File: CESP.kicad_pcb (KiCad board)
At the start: 2 copper layers, 55.9 x 44.7 mm, 9 parts

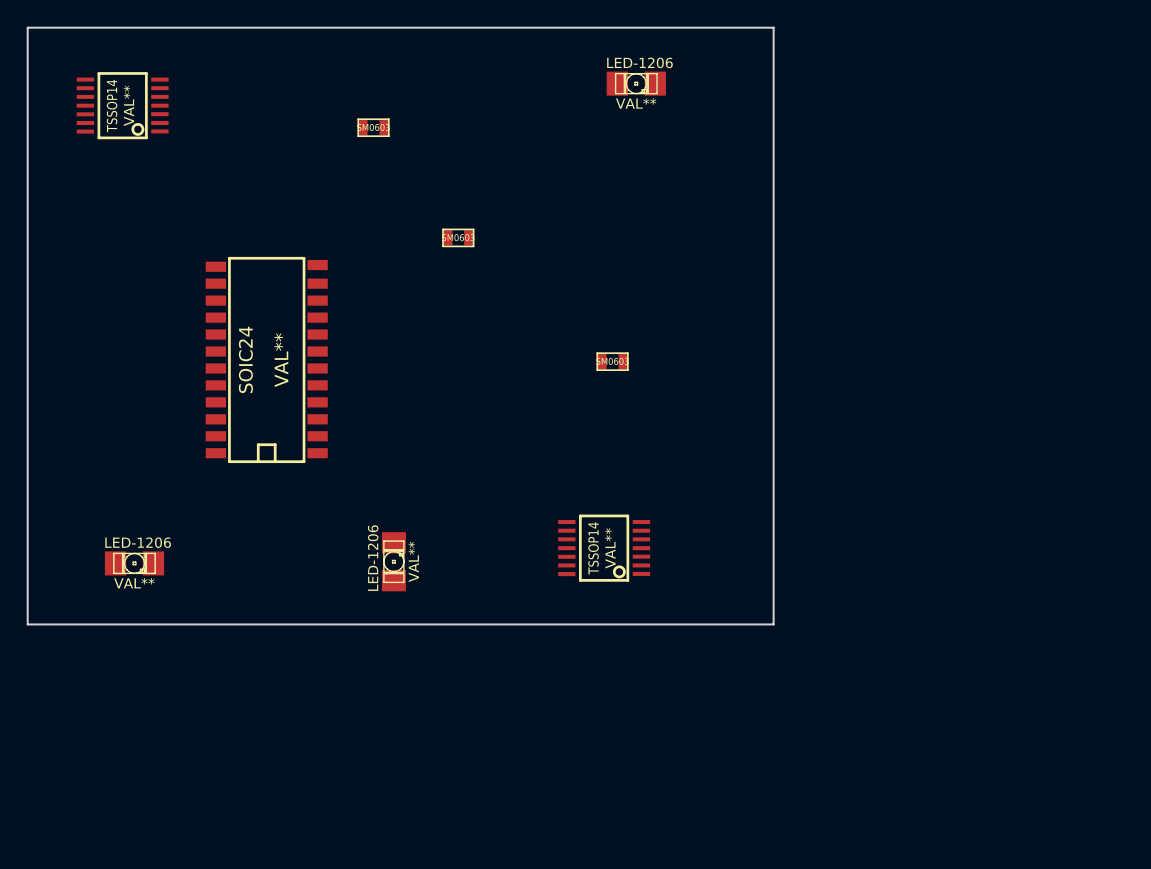
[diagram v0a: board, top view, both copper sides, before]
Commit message: Version1 commit
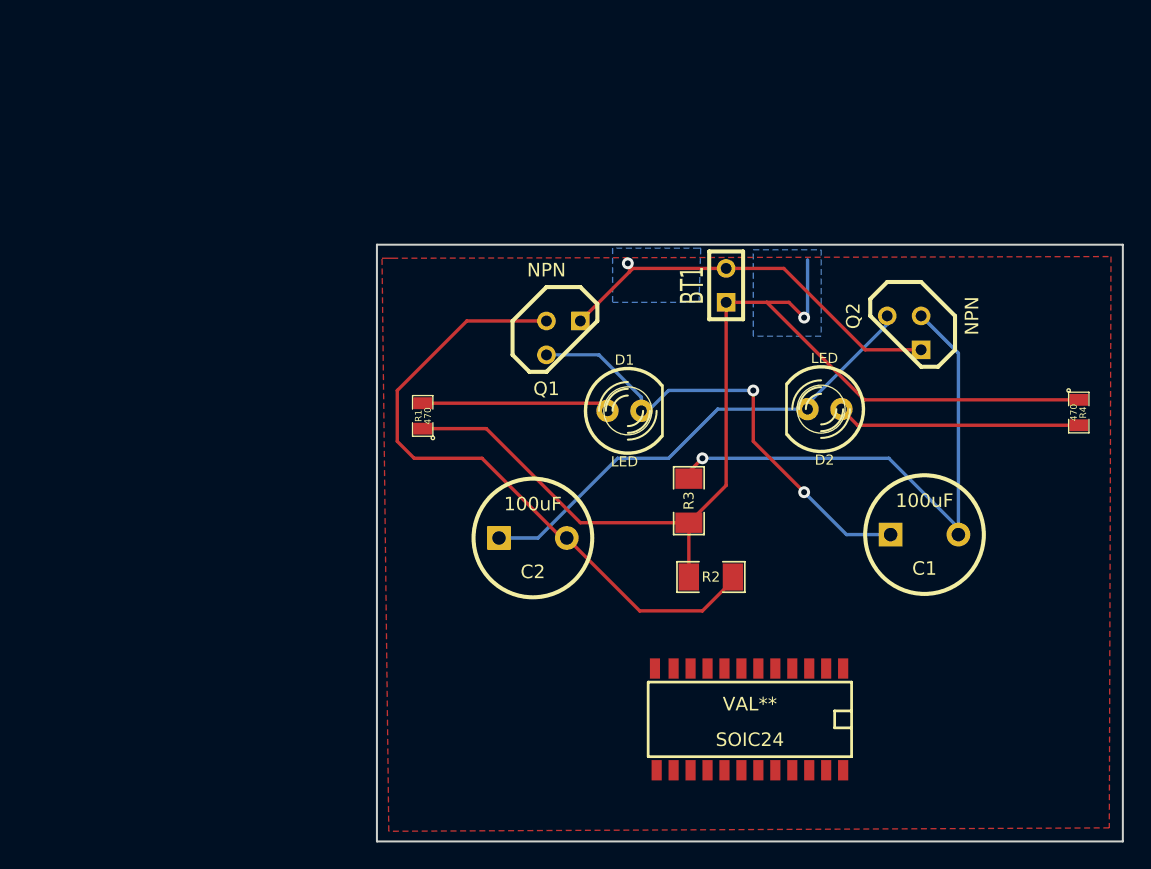
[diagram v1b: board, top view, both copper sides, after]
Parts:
- removed LED-1206 (x3): VAL**, LED-1206
- removed SM0603 (x3): Val**, SM0603
- removed TSSOP14 (x2): VAL**, TSSOP14
- added BT1: BATTERY, SIL-2, F.Cu at (208.3, 115.1)
- added C1: 100uF, C2V8, F.Cu at (223.1, 133.7)
- added C2: 100uF, C2V8, F.Cu at (193.8, 134.0)
- added D1: LED, LED-5MM, F.Cu at (200.7, 124.5)
- added D2: LED, LED-5MM, F.Cu at (215.6, 124.3)
- added Q1: NPN, TO92, F.Cu at (196.1, 119.0)
- added Q2: NPN, TO92, F.Cu at (221.6, 118.6)
- added R1: 470, SM0805, F.Cu at (185.5, 124.8)
- added R2: 10k, SM1206, F.Cu at (207.1, 136.9)
- added R3: 10k, SM1206, F.Cu at (205.5, 131.2)
- added R4: 470, SM0805, F.Cu at (234.7, 124.6)
- moved SOIC24 45.1 mm to (210.1, 147.6), turned to 180 degrees
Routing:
- net N-000008: track 0.00 -> 81.7 mm, vias 0 -> 1
- net N-000007: track 0.00 -> 48.8 mm
- net N-000002: track 0.00 -> 41.3 mm, vias 0 -> 1
- net N-000001: track 0.00 -> 36.6 mm
- net N-000003: track 0.00 -> 35.4 mm, vias 0 -> 2
- net N-000004: track 0.00 -> 30.5 mm, vias 0 -> 1
- net N-000006: track 0.00 -> 18.3 mm
- net N-000005: track 0.00 -> 14.1 mm
- added copper zone on F.Cu, net N-000001
- added copper zone on B.Cu, net N-000004
- added copper zone on B.Cu, net N-000008
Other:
- board text added: "2014"
- board text added: "Contextual"
- board text added: "Electronics"
- board text removed: "NOTE: THIS IS JUST A TEST BOARD REMOVE ALL COMPONENTS AND CREATE YOUR OWN INCLUDE SCHEMATIC HOOKUPS/NETLIST"
